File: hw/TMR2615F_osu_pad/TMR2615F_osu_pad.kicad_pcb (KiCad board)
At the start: 4 copper layers, 60 x 60 mm, 119 parts, among them J1 TYPE-C-31-M-12, J10 Conn_01x04, J2 TYPE-C-31-M-12, J3 Conn_01x02, J4 TYPE-C-31-M-12, J5 XY-SH1_0-4A61, J7 Conn_01x10, J8 Conn_01x06, J9 Conn_01x23, SW1 SKSGPAE010, SW2 SKSGPAE010, U1 CA-IS3722CHS, U10 TMR2615x, U11 CPG151101S11-16, U12 SK6812MINI-E, U13 TMR2615x, U14 CPG151101S11-16, U15 SK6812MINI-E, U16 TMR2615x, U17 CPG151101S11-16, U18 SK6812MINI-E, U19 TMR2615x, U2 SRV05-4A, U20 CPG151101S11-16, U21 SK6812MINI-E, U22 TMR2615x, U23 CPG151101S11-16, U24 SK6812MINI-E, U25 TMR2615x, U26 CPG151101S11-16, U27 SK6812MINI-E, U28 SRV05-4A, U3 TMUX1574RSVR, U4 LM66100DCK, U5 AP22653W6-7, U6 SRV05-4A, U7 AT32F405RBT7-7, U8 XC6206P332MR, U9 TPS7A4700, X1 X322512MSB4SI

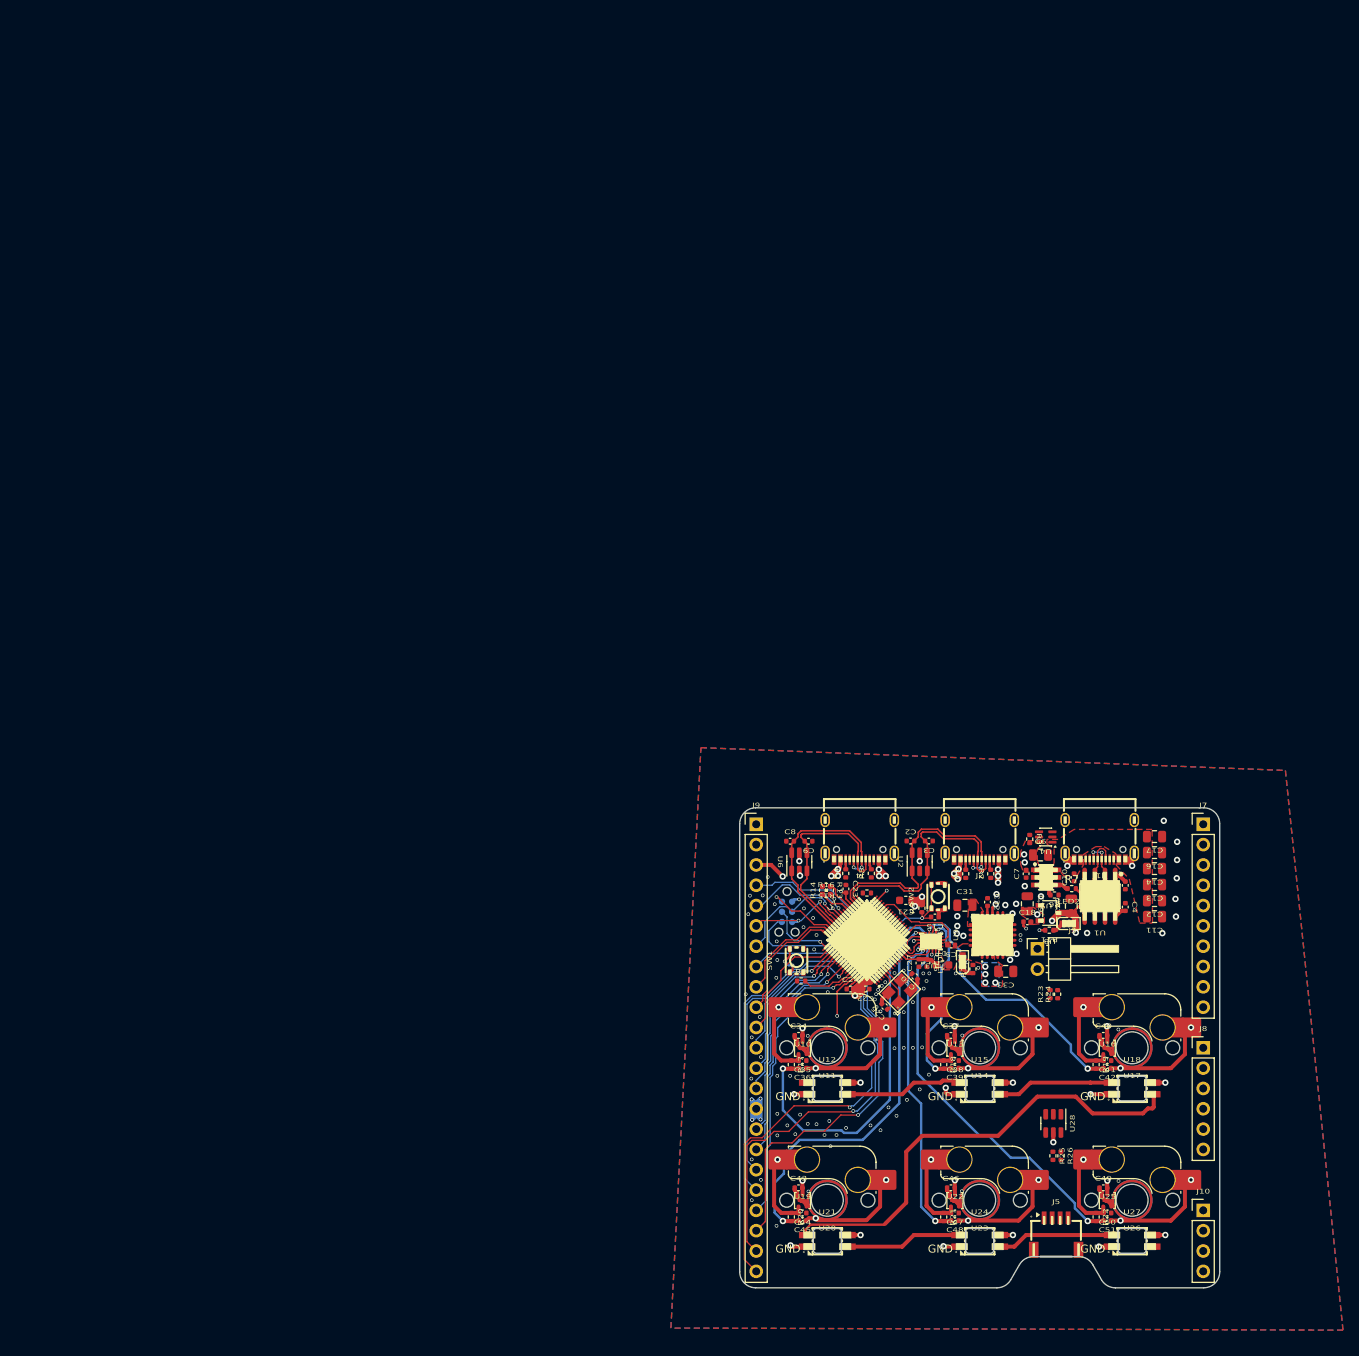
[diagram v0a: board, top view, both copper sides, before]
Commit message: before foob
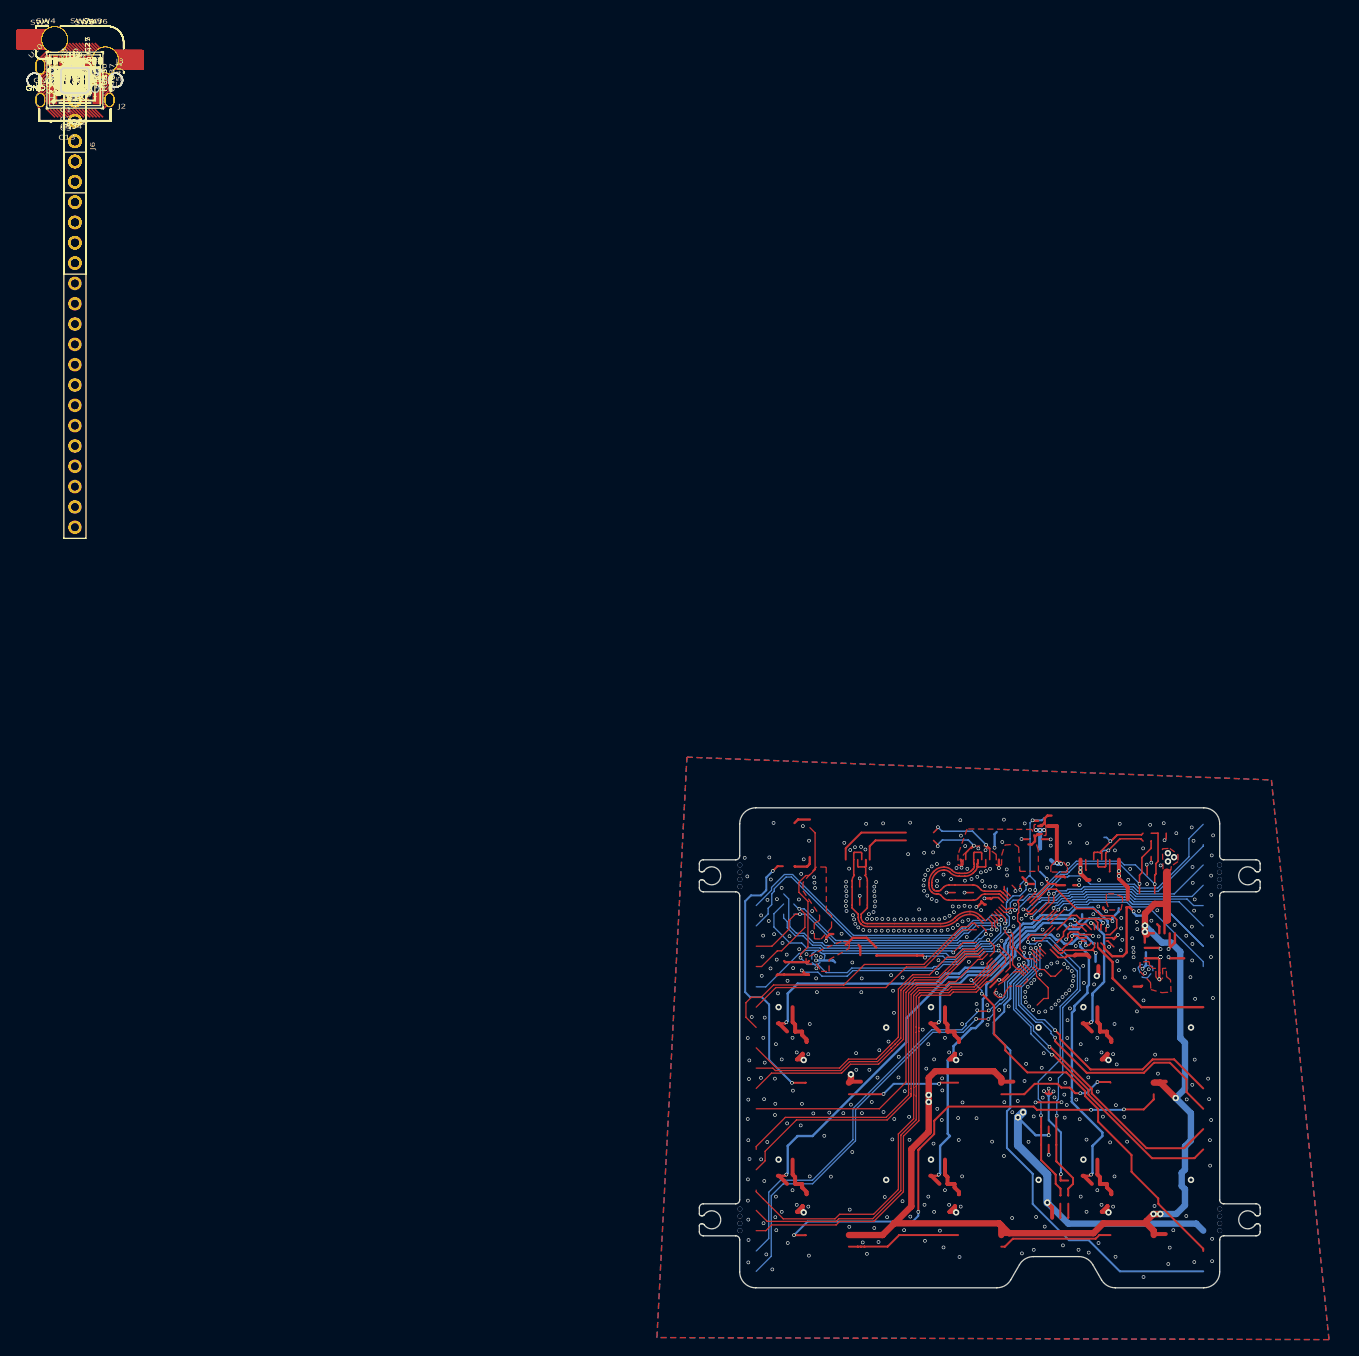
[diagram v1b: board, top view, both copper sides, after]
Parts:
- removed the C11 at (134.9, 104.6)
- removed the C13 at (134.9, 100.5)
- removed the C14 at (134.9, 98.5)
- removed the C16 at (134.9, 96.6)
- removed the C17 at (134.9, 94.5)
- removed the C35 at (91.0, 122.5)
- removed the C39 at (110.0, 123.5)
- removed the C47 at (110.0, 141.6)
- removed the C51 at (129.1, 142.6)
- removed the J3 at (120.3, 108.6)
- removed the R15 at (93.9, 100.8)
- removed the R16 at (93.9, 101.7)
- removed the R17 at (89.5, 123.0)
- removed the R18 at (108.6, 123.0)
- removed the R19 at (127.7, 123.0)
- removed the R20 at (89.5, 142.1)
- removed the R21 at (108.6, 142.1)
- removed the R22 at (127.7, 142.1)
- added C10, C34, C46, C54: CL10B473KB8NNNC, Capacitor_SMD:C_0603_1608Metric, F.Cu at (0.00, 0.00)
- added C2, C3, C6: CL21A226MAQNNNE, Capacitor_SMD:C_0805_2012Metric, F.Cu at (0.00, 0.00)
- added C28, C29, C40, C52, C56: CL05B104KB54PNC, Capacitor_SMD:C_0402_1005Metric, F.Cu at (0.00, 0.00)
- added C33, C37, C49, C53: 0402CG300J500NT, Capacitor_SMD:C_0402_1005Metric, F.Cu at (0.00, 0.00)
- added D1: 1N4148WS_T4, Diode_SMD:D_SOD-323_HandSoldering, F.Cu at (0.00, 0.00)
- added FID1, FID2, FID3: Fiducial, Fiducial:Fiducial_1mm_Mask2mm, F.Cu at (0.00, 0.00)
- added H1, H2, H3: MountingHole_Pad, MountingHole:MountingHole_2.2mm_M2_Pad_Via, F.Cu at (0.00, 0.00)
- added R1, R10, R2, R26, R4, R6, R9: 0402WGF1002TCE, Resistor_SMD:R_0402_1005Metric, F.Cu at (0.00, 0.00)
- added R12: 0402WGF5101TCE, Resistor_SMD:R_0402_1005Metric, F.Cu at (0.00, 0.00)
- added R27, R3: 0402WGF1200TCE, Resistor_SMD:R_0402_1005Metric, F.Cu at (0.00, 0.00)
- added R29, R30, R31, R32, R33, R34: 0402WGF3300TCE, Resistor_SMD:R_0402_1005Metric, F.Cu at (0.00, 0.00)
- added TP1, TP10, TP11, TP12, TP13, TP14, TP15, TP16, TP17, TP18, TP19, TP2, TP20, TP21, TP22, TP3, TP4, TP5, TP6, TP7, TP8, TP9: TestPoint, TestPoint:TestPoint_Pad_D1.0mm, B.Cu at (0.00, 0.00)
- added U12: SK6812MINI-E, LED__C:LED-SMD_4P-L3.2-W2.8-LS5.9_SK6812MINI-E, F.Cu at (0.00, 0.00)
- added U7: LM66100DCK, Package_TO_SOT_SMD:SOT-363_SC-70-6, F.Cu at (0.00, 0.00)
- C1, C4, C5: value CL05B104KB54PNC -> CL21A226MAQNNNE; footprint Capacitor_SMD:C_0402_1005Metric -> Capacitor_SMD:C_0805_2012Metric
- C12: value CL21A226MAQNNNE -> CL21A106KAYNNNE
- C36, C48: value 0402CG300J500NT -> CL05B104KB54PNC
- C38, C50: value CL05B104KB54PNC -> CL10B473KB8NNNC; footprint Capacitor_SMD:C_0402_1005Metric -> Capacitor_SMD:C_0603_1608Metric
- C41: value CL05B104KB54PNC -> 0402CG300J500NT
- C42: value 0402CG300J500NT -> CL10B473KB8NNNC; footprint Capacitor_SMD:C_0402_1005Metric -> Capacitor_SMD:C_0603_1608Metric
- R13: value 0402WGF0000TCE -> 0402WGF5101TCE
- R14: value 0402WGF0000TCE -> 0402WGF1200TCE
- R7: value 0402WGF1002TCE -> 0402WGF1200TCE
- R8: value 0402WGF3301TCE -> 0402WGF3300TCE
- U1: value CA-IS3722CHS -> SRV05-4A; footprint Isolator__C:SOIC-8_L4.9-W3.9-P1.27-LS6.0-BL -> Diode__C:SOT-23-6
- moved J8 199.6 mm to (0.00, 0.00)
- moved U24 196.2 mm to (0.00, 0.00)
- moved SW8 192.5 mm to (0.00, 0.00)
- moved C50 191.6 mm to (0.00, 0.00), turned to 0 degrees
- moved U23 190.4 mm to (0.00, 0.00)
- moved J4 189.3 mm to (0.00, 0.00)
- moved C55 188.9 mm to (0.00, 0.00)
- moved J7 185.8 mm to (0.00, 0.00)
- moved U22 184.0 mm to (0.00, 0.00)
- moved U18 182.6 mm to (0.00, 0.00)
- moved R16 182.4 mm to (0.00, 0.00), turned to 0 degrees
- moved R21 181.7 mm to (0.00, 0.00), turned to 0 degrees
- moved C48 180.1 mm to (0.00, 0.00), turned to 0 degrees
- moved SW7 180.0 mm to (0.00, 0.00)
- moved SW5 179.1 mm to (0.00, 0.00)
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- renumbered C10 to C11, C31 to C13, C32 to C14, C8 to C15, C9 to C16, C2 to C17, C3 to C18, C18 to C19, C19 to C20, C20 to C21, C26 to C22, C27 to C23, C21 to C24, C22 to C25, C23 to C26, C24 to C27, C15 to C30, C25 to C31, C30 to C32, C34 to C35, C37 to C39, C40 to C43, C43 to C47, C46 to C51, C49 to C55, C6 to C7, C7 to C8, C33 to C9, J4 to J2, J2 to J3, J5 to J4, J7 to J5, J9 to J6, J8 to J7, J10 to J8, J6 to J9, R6 to R11, R24 to R15, R26 to R16, R4 to R17, R5 to R18, R1 to R19, R2 to R20, R25 to R21, R23 to R22, R10 to R23, R11 to R24, R12 to R25, R9 to R28, R3 to R5, U11 to SW3, U14 to SW4, U17 to SW5, U20 to SW6, U23 to SW7, U26 to SW8, U7 to U10, U3 to U11, U10 to U13, U12 to U14, U13 to U15, U15 to U16, U16 to U17, U4 to U2, U21 to U20, U22 to U21, U24 to U22, U25 to U23, U27 to U24, U5 to U3, U9 to U4, U6 to U5, U2 to U6, U28 to U9
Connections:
- net /IO10 renamed /LM_ST
- C1 pad 2: Net-(U1-VDDA) -> +5V
- C11 pad 2: /VBUS_B -> VBUS_B
- C12 pad 1: GND -> VBUS_B
- C12 pad 2: /VBUS_B -> GND
- C36 pad 2: /TMUX_S1A -> +5V
- C38 pad 2: Net-(U13-VOUT) (its old number) -> /TMUX_S1B
- C4 pad 2: Net-(U1-VDDB) -> +5V
- C44 pad 2: Net-(U19-VOUT) -> +5V
- C45 pad 2: /TMUX_S2B -> Net-(U19-VOUT)
- C48 pad 2: /TMUX_S3A -> +5V
- C5 pad 2: +3.3VA -> +5V
- C50 pad 2: Net-(U25-VOUT) -> /TMUX_S3A
- C7 pad 1: +5V -> VBUS_HOST
- C8 pad 2: +5V -> VBUS_HOST
- J1 pad A4B9: /VBUS_B -> VBUS_B
- J1 pad A5: unconnected-(J1-CC1-PadA5) -> Net-(J1-CC1)
- J1 pad B4A9: /VBUS_B -> VBUS_B
- J1 pad B5: unconnected-(J1-CC2-PadB5) -> Net-(J1-CC2)
- J2 pad A4B9: +5V -> unconnected-(J2-VBUS-PadA4B9)
- J2 pad B4A9: +5V -> unconnected-(J2-VBUS-PadB4A9)
- J3 pad A4B9: +5V -> VBUS_HOST
- J3 pad B4A9: +5V -> VBUS_HOST
- J5 pad 10: /TMUX_S4A -> /TMUX_S4B
- J5 pad 9: /TMUX_S4B -> GND
- J6 pad 10: /I2C2_SCL -> /I2C2_SDA
- J6 pad 11: /SPI3_CS -> /I2C2_SCL
- J6 pad 12: /SPI3_SCK -> /SPI3_CS
- J6 pad 13: /SPI3_MISO -> /SPI3_SCK
- J6 pad 14: /SPI3_MOSI -> /SPI3_MISO
- J6 pad 15: GND -> /SPI3_MOSI
- J6 pad 16: /IO1 -> GND
- J6 pad 17: /IO2 -> /IO1
- J6 pad 18: /IO3 -> /IO2
- J6 pad 19: /IO4 -> /IO3
- J6 pad 2: +5V -> GND
- J6 pad 20: /IO5 -> /IO4
- J6 pad 21: /IO6 -> /IO5
- J6 pad 22: /IO7 -> /IO6
- J6 pad 23: /IO8 -> /IO7
- J6 pad 3: +3.3V -> +5V
- J6 pad 4: /UART8_TX -> +3.3V
- J6 pad 5: /UART8_RX -> /UART8_TX
- J6 pad 6: /USART1_RX -> /UART8_RX
- J6 pad 7: /USART1_TX -> /USART1_RX
- J6 pad 8: /USART1_CK -> /USART1_TX
- J6 pad 9: /I2C2_SDA -> /USART1_CK
- R13 pad 1: Net-(U7-PC6) -> GND
- R13 pad 2: /UART7_TX -> Net-(J1-CC1)
- R14 pad 1: Net-(U7-PC7) -> Net-(R14-Pad1)
- R14 pad 2: /UART7_RX -> +3.3V
- R15 pad 2: Net-(J3-Pin_2) -> Net-(R14-Pad1)
- R22 pad 2: Net-(J3-Pin_2) -> Net-(R14-Pad1)
- R5 pad 2: +5V -> +3.3V
- R7 pad 1: /IO9 -> Net-(J1-DP1)
- R7 pad 2: +3.3V -> /UART7_TX
- R8 pad 1: GND -> /TMUX_S4A
- R8 pad 2: /BOOT -> Net-(C10-Pad2)
- SW4 pad 2: Net-(U13-VOUT) (its old number) -> Net-(U15-VOUT)
- SW8 pad 2: Net-(U25-VOUT) -> Net-(U23-VOUT)
- U1 pad 1: Net-(U1-VDDA) -> /UART7_RX
- U1 pad 2: Net-(J1-DP1) -> GND
- U1 pad 3: Net-(J1-DN1) -> /UART7_TX
- U1 pad 4: GND -> /UART7_TX
- U1 pad 5: GND -> +3.3V
- U10 pad 2: /IO6 -> /PW_PSTRH
- U10 pad 29: /IO9 -> /AP_FAULT
- U10 pad 3: /IO7 -> /IO6
- U10 pad 37: Net-(U7-PC6) -> /UART7_RX
- U10 pad 38: Net-(U7-PC7) -> /UART7_TX
- U10 pad 4: /IO8 -> /IO7
- U10 pad 62: /DIN -> Net-(U10-PB9)
- U11 pad 13: +3.3VA -> GND
- U15 pad 1: Net-(U13-VOUT) (its old number) -> Net-(U15-VOUT)
- U2 pad 1: /VBUS_B -> VBUS_B
- U2 pad 3: GND -> +5V
- U23 pad 1: Net-(U25-VOUT) -> Net-(U23-VOUT)
- U3 pad 1: +5V -> VBUS_HOST
- U3 pad 3: +5V -> /PW_PSTRH
- U3 pad 4: /IO9 -> /AP_FAULT
- U3 pad 6: /VBUS_B -> VBUS_B
- U9 pad 1: /I2C1_SCL -> /I2C1_SDA
- U9 pad 3: /I2C1_SDA -> /I2C1_SCL
- U9 pad 4: /I2C1_SDA -> /I2C1_SCL
- U9 pad 5: +5V -> +3.3V
- U9 pad 6: /I2C1_SCL -> /I2C1_SDA
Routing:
- net +5V: track 29.5 -> 254.4 mm, vias 26 -> 19
- net +3.3V: track 30.9 -> 176.1 mm, vias 9 -> 17
- net GND: track 167.0 -> 30.9 mm, vias 134 -> 473
- net /I2C3_SCL: track 0.00 -> 68.5 mm, vias 0 -> 1
- net /IO8: track 54.9 -> 0.00 mm, vias 2 -> 0
- net /I2C3_SDA: track 0.00 -> 52.7 mm, vias 0 -> 2
- net Net-(U10-PB9): track 0.00 -> 49.6 mm, vias 0 -> 2
- net /I2C1_SDA: track 0.00 -> 43.5 mm, vias 0 -> 2
- net /ADC1_IN11: track 0.00 -> 42.8 mm, vias 0 -> 2
- net /ADC1_IN10: track 0.00 -> 42.3 mm, vias 0 -> 2
- net /I2C1_SCL: track 0.00 -> 41.7 mm, vias 0 -> 2
- net /ADC1_IN12: track 0.00 -> 40.4 mm, vias 0 -> 2
- net /ADC1_IN5: track 0.00 -> 39.2 mm, vias 0 -> 1
- net /ADC1_IN13: track 0.00 -> 38.2 mm, vias 0 -> 2
- net /UART7_TX: track 0.77 -> 32.8 mm, vias 1 -> 2
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- added copper zone on B.Cu, net +3.3V
- added copper zone on F.Cu, net +3.3V
- added copper zone on In2.Cu, net +3.3V
- added copper zone on In2.Cu, net +5V
- added copper zone on F.Cu, net Net-(C10-Pad2)
- added copper zone on F.Cu, net VBUS_B
- added copper zone on In2.Cu, net VBUS_B
- added copper zone on F.Cu, net VBUS_HOST
- removed copper zone on In1.Cu, net +3.3VA
- removed copper zone on F.Cu, net /VBUS_B
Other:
- board size 60 x 60 mm -> 70.1 x 60 mm
